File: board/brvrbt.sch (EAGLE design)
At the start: 9 parts

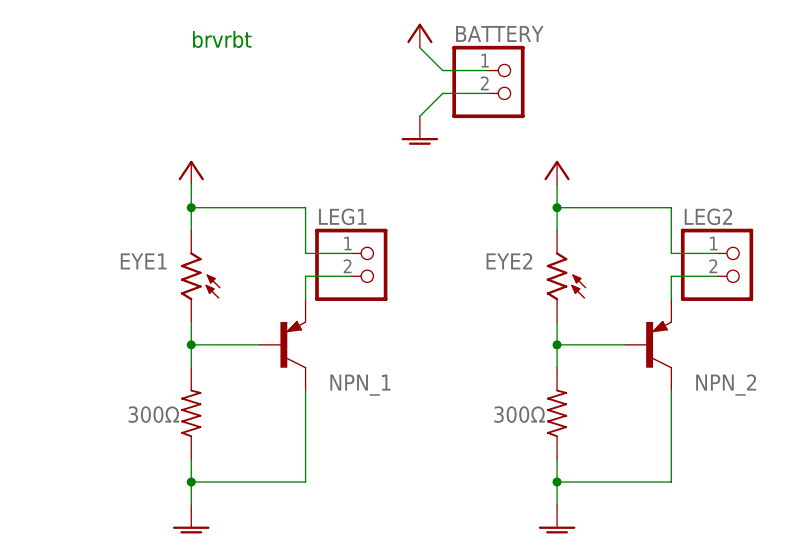
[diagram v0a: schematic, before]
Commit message: layout
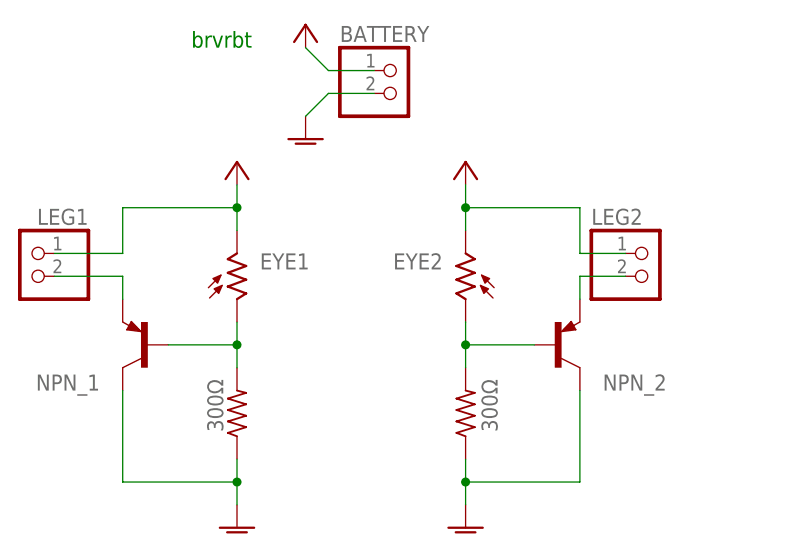
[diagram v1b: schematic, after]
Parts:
- R1, R2: device adafruit:R-US_0207/12 -> adafruit:R-US_0207/7
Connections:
- net AGND renamed GND
- net N$1 renamed BASE_2
- net N$2 renamed COLLECTOR_2
- net N$3 renamed BASE_1
- net N$4 renamed COLLECTOR_1
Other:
- moved on the sheet: BATTERY, EYE1, EYE2, LEG1, LEG2, NPN_1, NPN_2
